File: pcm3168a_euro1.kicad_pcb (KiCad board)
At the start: 2 copper layers, 196 x 128.4 mm, 213 parts, among them J1 Conn_02x04_Odd_Even, J10 Conn_Coaxial, J11 Conn_Coaxial, J12 Conn_Coaxial, J13 Conn_Coaxial, J14 Conn_Coaxial, J15 Conn_Coaxial, J16 Conn_Coaxial, J17 ACJS-MV35-3, J18 Conn_02x08_Odd_Even, J19 Conn_Coaxial, J2 Conn_02x04_Odd_Even, J20 ACJS-MV35-3, J21 ACJS-MV35-3, J22 ACJS-MV35-3, J3 Conn_02x04_Odd_Even, J4 Conn_02x04_Odd_Even, J5 Conn_02x04_Odd_Even, J6 Conn_Coaxial, J7 Conn_Coaxial, J8 Conn_01x02_Pin, J9 Conn_Coaxial, U1 PCM3168APAPR, U10 74LVC1G17, U11 OPA1637, U12 TLV1117-33, U13 OPA1637, U14 OPA1637, U15 OPA1637, U2 74LVC1G17, U3 74LVC1G17, U4 74LVC1G17, U5 74LVC1G17, U6 74LVC1G17, U7 74LVC1G17, U8 74LVC1G17, U9 74LVC1G17, Y1 SG-210STF 24.5760ML0

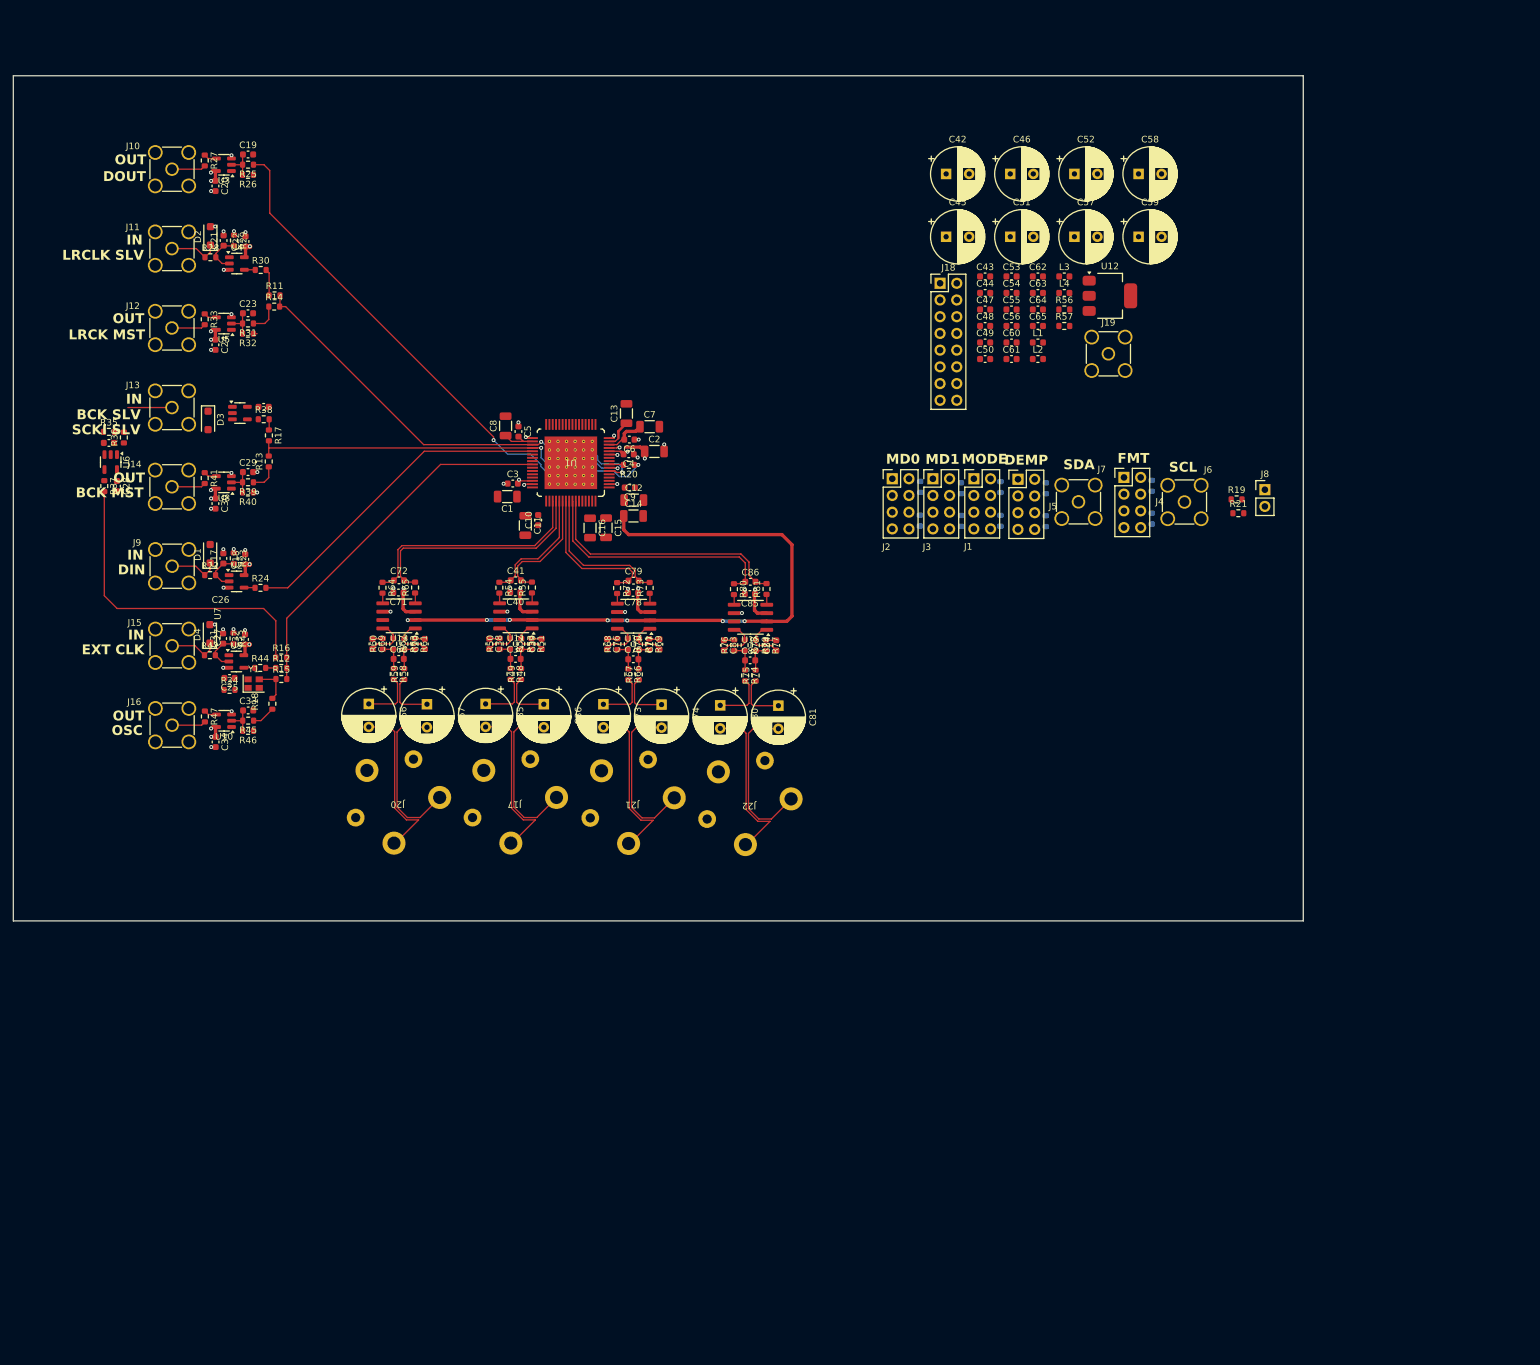
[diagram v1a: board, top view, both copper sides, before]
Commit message: WIP layout
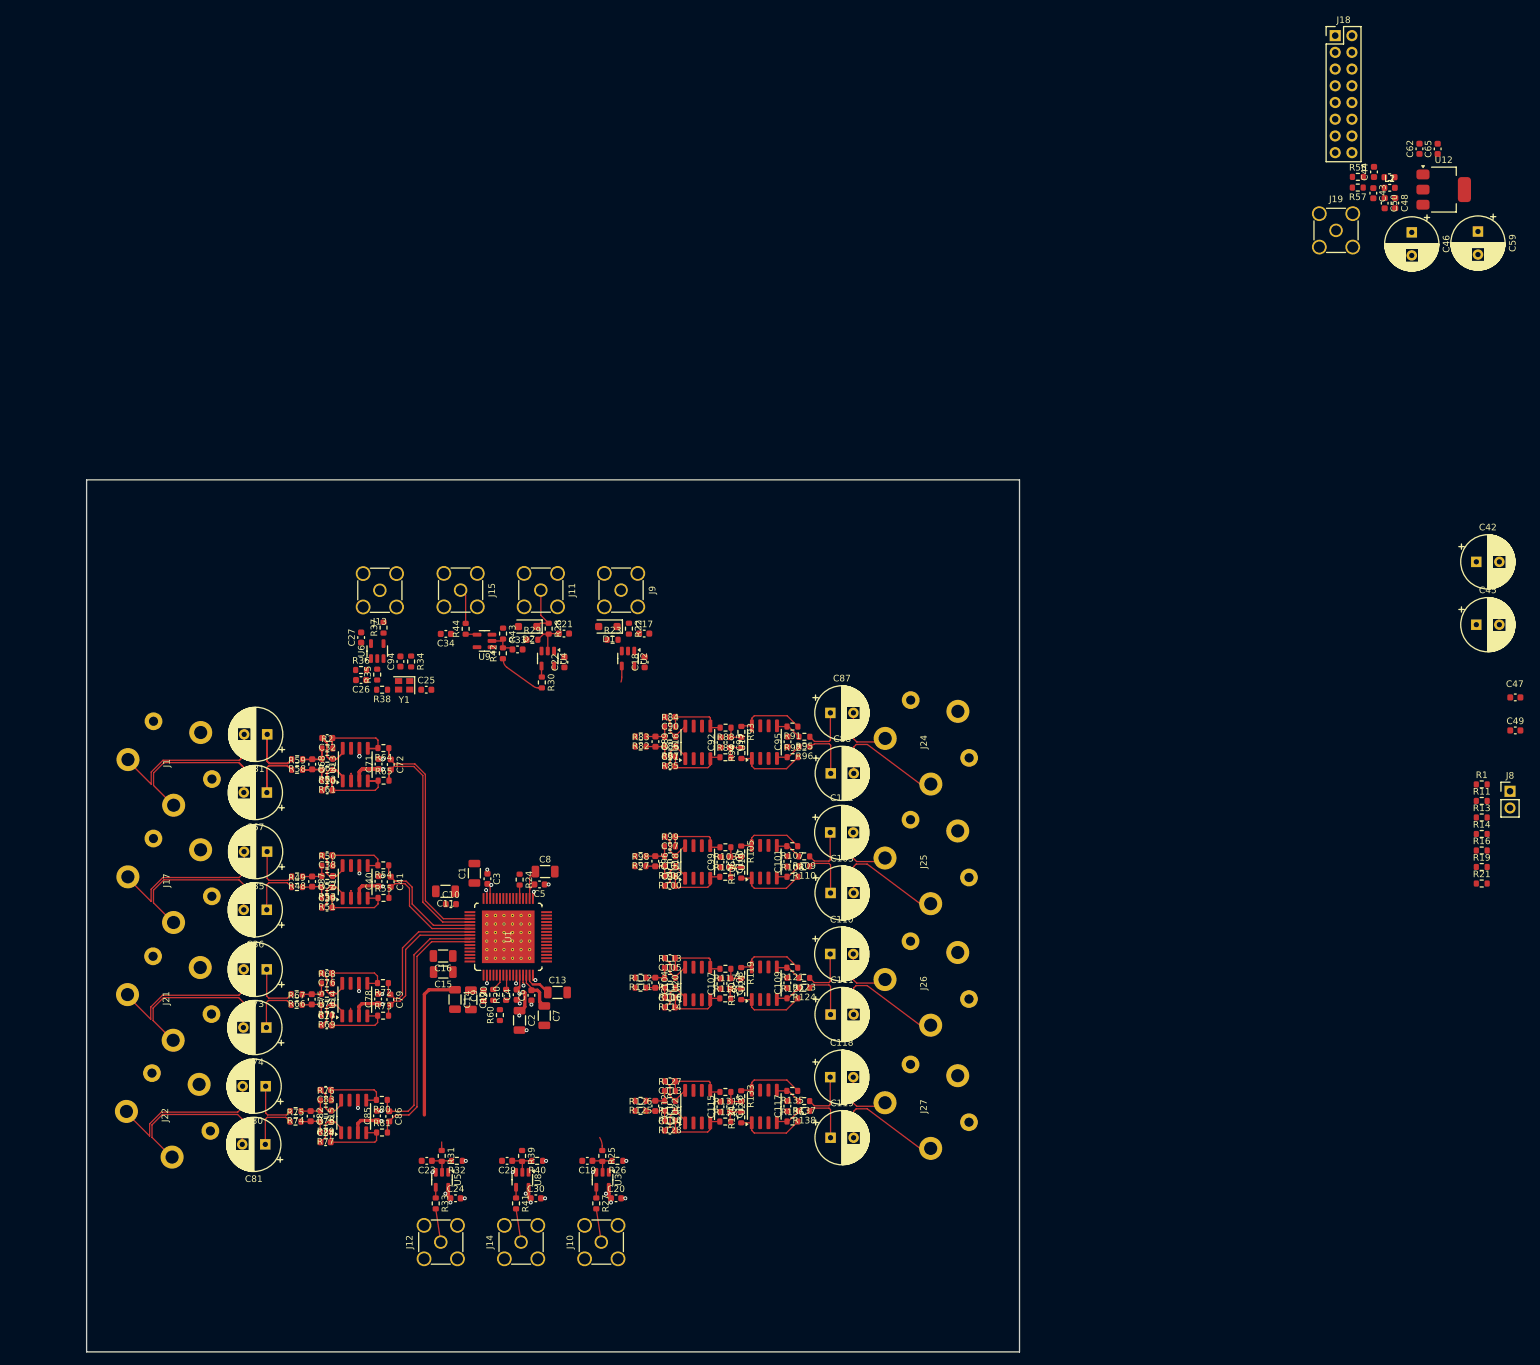
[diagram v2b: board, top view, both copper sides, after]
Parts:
- removed C28: 100nF, Capacitor_SMD:C_0603_1608Metric
- removed C51, C52, C57, C58, C66: C_Polarized_Small, Capacitor_THT:CP_Radial_D8.0mm_P3.50mm
- removed C53, C54, C55, C56, C60, C61, C63, C64: C_Small, Capacitor_SMD:C_0603_1608Metric
- removed C69: 1n, Capacitor_SMD:C_0603_1608Metric
- removed D3, D4: D_Zener_Small, Diode_SMD:D_SOD-123F
- removed J16, J6, J7: Conn_Coaxial, Connector_Coaxial:SMA_Amphenol_901-144_Vertical
- removed J2, J3, J4, J5: Conn_02x04_Odd_Even, Connector_PinHeader_2.54mm:PinHeader_2x04_P2.54mm_Vertical
- removed J20: ACJS-MV35-3, pcm3168a_euro1:Amphenol_ACJS
- removed L3, L4: L_Ferrite_Small, Inductor_SMD:L_0603_1608Metric
- removed R10, R3, R4, R5, R6, R7, R8, R9: 220k 5%, Resistor_SMD:R_0603_1608Metric
- removed R12, R15, R17, R18, R45: 0, Resistor_SMD:R_0603_1608Metric
- removed R46: R_Small, Resistor_SMD:R_0603_1608Metric
- removed R47: 22, Resistor_SMD:R_0603_1608Metric
- removed U10, U7: 74LVC1G17, Package_TO_SOT_SMD:SOT-23-5
- added C100: 39n, Capacitor_SMD:C_0603_1608Metric, F.Cu at (160.4, 142.6)
- added C101: 100nF, Capacitor_SMD:C_0603_1608Metric, F.Cu at (169.1, 142.5)
- added C102: C_Polarized_Small, Capacitor_THT:CP_Radial_D8.0mm_P3.50mm, F.Cu at (175.6, 138.1)
- added C103: C_Polarized_Small, Capacitor_THT:CP_Radial_D8.0mm_P3.50mm, F.Cu at (175.7, 147.3)
- added C104: 6.8n, Capacitor_SMD:C_0603_1608Metric, F.Cu at (149.1, 160.9)
- added C105: 1n, Capacitor_SMD:C_0603_1608Metric, F.Cu at (151.3, 157.2)
- added C106: 1n, Capacitor_SMD:C_0603_1608Metric, F.Cu at (151.3, 164.7)
- added C107: 100nF, Capacitor_SMD:C_0603_1608Metric, F.Cu at (159.0, 161.1)
- added C108: 39n, Capacitor_SMD:C_0603_1608Metric, F.Cu at (160.4, 161.0)
- added C109: 100nF, Capacitor_SMD:C_0603_1608Metric, F.Cu at (169.1, 161.0)
- added C110: C_Polarized_Small, Capacitor_THT:CP_Radial_D8.0mm_P3.50mm, F.Cu at (175.6, 156.6)
- added C111: C_Polarized_Small, Capacitor_THT:CP_Radial_D8.0mm_P3.50mm, F.Cu at (175.7, 165.8)
- added C112: 6.8n, Capacitor_SMD:C_0603_1608Metric, F.Cu at (149.1, 179.7)
- added C113: 1n, Capacitor_SMD:C_0603_1608Metric, F.Cu at (151.3, 175.9)
- added C114: 1n, Capacitor_SMD:C_0603_1608Metric, F.Cu at (151.3, 183.4)
- added C115: 100nF, Capacitor_SMD:C_0603_1608Metric, F.Cu at (159.0, 179.8)
- added C116: 39n, Capacitor_SMD:C_0603_1608Metric, F.Cu at (160.4, 179.8)
- added C117: 100nF, Capacitor_SMD:C_0603_1608Metric, F.Cu at (169.1, 179.7)
- added C118: C_Polarized_Small, Capacitor_THT:CP_Radial_D8.0mm_P3.50mm, F.Cu at (175.6, 175.3)
- added C119: C_Polarized_Small, Capacitor_THT:CP_Radial_D8.0mm_P3.50mm, F.Cu at (175.7, 184.5)
- added C87: C_Polarized_Small, Capacitor_THT:CP_Radial_D8.0mm_P3.50mm, F.Cu at (175.7, 119.9)
- added C88: C_Polarized_Small, Capacitor_THT:CP_Radial_D8.0mm_P3.50mm, F.Cu at (175.7, 129.1)
- added C89: 6.8n, Capacitor_SMD:C_0603_1608Metric, F.Cu at (149.1, 124.3)
- added C90: 1n, Capacitor_SMD:C_0603_1608Metric, F.Cu at (151.3, 120.5)
- added C91: 1n, Capacitor_SMD:C_0603_1608Metric, F.Cu at (151.3, 128.0)
- added C92: 100nF, Capacitor_SMD:C_0603_1608Metric, F.Cu at (159.0, 124.4)
- added C93: 39n, Capacitor_SMD:C_0603_1608Metric, F.Cu at (160.5, 124.4)
- added C94: 4.7uF, Capacitor_SMD:C_0603_1608Metric, F.Cu at (110.3, 112.1)
- added C95: 100nF, Capacitor_SMD:C_0603_1608Metric, F.Cu at (169.1, 124.3)
- added C96: 6.8n, Capacitor_SMD:C_0603_1608Metric, F.Cu at (149.1, 142.5)
- added C97: 1n, Capacitor_SMD:C_0603_1608Metric, F.Cu at (151.3, 138.7)
- added C98: 1n, Capacitor_SMD:C_0603_1608Metric, F.Cu at (151.3, 146.2)
- added C99: 100nF, Capacitor_SMD:C_0603_1608Metric, F.Cu at (159.0, 142.6)
- added J24: ACJS-MV35-3, pcm3168a_euro1:Amphenol_ACJS, F.Cu at (190.4, 124.4)
- added J25: ACJS-MV35-3, pcm3168a_euro1:Amphenol_ACJS, F.Cu at (190.3, 142.5)
- added J26: ACJS-MV35-3, pcm3168a_euro1:Amphenol_ACJS, F.Cu at (190.3, 161.0)
- added J27: ACJS-MV35-3, pcm3168a_euro1:Amphenol_ACJS, F.Cu at (190.3, 179.7)
- added R100: 1.1k, Resistor_SMD:R_0603_1608Metric, F.Cu at (151.3, 144.7)
- added R101: 560, Resistor_SMD:R_0603_1608Metric, F.Cu at (151.3, 141.7)
- added R102: 560, Resistor_SMD:R_0603_1608Metric, F.Cu at (151.3, 143.2)
- added R103: 47, Resistor_SMD:R_0603_1608Metric, F.Cu at (159.7, 140.3)
- added R104: 47, Resistor_SMD:R_0603_1608Metric, F.Cu at (159.7, 144.8)
- added R105: 1.1k, Resistor_SMD:R_0603_1608Metric, F.Cu at (162.1, 141.0)
- added R106: 1.1k, Resistor_SMD:R_0603_1608Metric, F.Cu at (162.1, 144.2)
- added R107: 1.1k, Resistor_SMD:R_0603_1608Metric, F.Cu at (169.9, 140.2)
- added R108: 1.1k, Resistor_SMD:R_0603_1608Metric, F.Cu at (169.9, 144.8)
- added R109: 120, Resistor_SMD:R_0603_1608Metric, F.Cu at (171.7, 141.7)
- added R110: 120, Resistor_SMD:R_0603_1608Metric, F.Cu at (171.7, 143.2)
- added R111: 1.1k, Resistor_SMD:R_0603_1608Metric, F.Cu at (146.8, 160.2)
- added R112: 1.1k, Resistor_SMD:R_0603_1608Metric, F.Cu at (146.8, 161.7)
- added R113: 1.1k, Resistor_SMD:R_0603_1608Metric, F.Cu at (151.3, 158.7)
- added R114: 1.1k, Resistor_SMD:R_0603_1608Metric, F.Cu at (151.3, 163.2)
- added R115: 560, Resistor_SMD:R_0603_1608Metric, F.Cu at (151.3, 160.2)
- added R116: 560, Resistor_SMD:R_0603_1608Metric, F.Cu at (151.3, 161.7)
- added R117: 47, Resistor_SMD:R_0603_1608Metric, F.Cu at (159.7, 158.8)
- added R118: 47, Resistor_SMD:R_0603_1608Metric, F.Cu at (159.7, 163.3)
- added R119: 1.1k, Resistor_SMD:R_0603_1608Metric, F.Cu at (162.1, 159.4)
- added R120: 1.1k, Resistor_SMD:R_0603_1608Metric, F.Cu at (162.1, 162.7)
- added R121: 1.1k, Resistor_SMD:R_0603_1608Metric, F.Cu at (169.9, 158.6)
- added R122: 1.1k, Resistor_SMD:R_0603_1608Metric, F.Cu at (169.9, 163.3)
- added R123: 120, Resistor_SMD:R_0603_1608Metric, F.Cu at (171.7, 160.2)
- added R124: 120, Resistor_SMD:R_0603_1608Metric, F.Cu at (171.7, 161.7)
- added R125: 1.1k, Resistor_SMD:R_0603_1608Metric, F.Cu at (146.8, 178.9)
- added R126: 1.1k, Resistor_SMD:R_0603_1608Metric, F.Cu at (146.8, 180.4)
- added R127: 1.1k, Resistor_SMD:R_0603_1608Metric, F.Cu at (151.3, 177.4)
- added R128: 1.1k, Resistor_SMD:R_0603_1608Metric, F.Cu at (151.3, 181.9)
- added R129: 560, Resistor_SMD:R_0603_1608Metric, F.Cu at (151.3, 178.9)
- added R130: 560, Resistor_SMD:R_0603_1608Metric, F.Cu at (151.3, 180.4)
- added R131: 47, Resistor_SMD:R_0603_1608Metric, F.Cu at (159.7, 177.5)
- added R132: 47, Resistor_SMD:R_0603_1608Metric, F.Cu at (159.7, 182.0)
- added R133: 1.1k, Resistor_SMD:R_0603_1608Metric, F.Cu at (162.1, 178.2)
- added R134: 1.1k, Resistor_SMD:R_0603_1608Metric, F.Cu at (162.1, 181.4)
- added R135: 1.1k, Resistor_SMD:R_0603_1608Metric, F.Cu at (169.9, 177.4)
- added R136: 1.1k, Resistor_SMD:R_0603_1608Metric, F.Cu at (169.9, 182.0)
- added R137: 120, Resistor_SMD:R_0603_1608Metric, F.Cu at (171.7, 178.9)
- added R138: 120, Resistor_SMD:R_0603_1608Metric, F.Cu at (171.7, 180.4)
- added R82: 1.1k, Resistor_SMD:R_0603_1608Metric, F.Cu at (146.8, 123.5)
- added R83: 1.1k, Resistor_SMD:R_0603_1608Metric, F.Cu at (146.8, 125.0)
- added R84: 1.1k, Resistor_SMD:R_0603_1608Metric, F.Cu at (151.3, 122.0)
- added R85: 1.1k, Resistor_SMD:R_0603_1608Metric, F.Cu at (151.3, 126.5)
- added R86: 560, Resistor_SMD:R_0603_1608Metric, F.Cu at (151.3, 123.5)
- added R87: 560, Resistor_SMD:R_0603_1608Metric, F.Cu at (151.3, 125.0)
- added R88: 47, Resistor_SMD:R_0603_1608Metric, F.Cu at (159.7, 122.2)
- added R89: 47, Resistor_SMD:R_0603_1608Metric, F.Cu at (159.7, 126.7)
- added R90: 22, Resistor_SMD:R_0603_1608Metric, F.Cu at (124.4, 162.8)
- added R91: 1.1k, Resistor_SMD:R_0603_1608Metric, F.Cu at (169.9, 122.0)
- added R92: 1.1k, Resistor_SMD:R_0603_1608Metric, F.Cu at (169.9, 126.7)
- added R93: 1.1k, Resistor_SMD:R_0603_1608Metric, F.Cu at (162.1, 122.8)
- added R94: 1.1k, Resistor_SMD:R_0603_1608Metric, F.Cu at (162.1, 126.0)
- added R95: 120, Resistor_SMD:R_0603_1608Metric, F.Cu at (171.7, 123.6)
- added R96: 120, Resistor_SMD:R_0603_1608Metric, F.Cu at (171.7, 125.1)
- added R97: 1.1k, Resistor_SMD:R_0603_1608Metric, F.Cu at (146.8, 141.7)
- added R98: 1.1k, Resistor_SMD:R_0603_1608Metric, F.Cu at (146.8, 143.2)
- added R99: 1.1k, Resistor_SMD:R_0603_1608Metric, F.Cu at (151.3, 140.2)
- added U16: OPA1637, Package_SO:SOIC-8_3.9x4.9mm_P1.27mm, F.Cu at (155.5, 124.4)
- added U17: OPA1637, Package_SO:SOIC-8_3.9x4.9mm_P1.27mm, F.Cu at (165.6, 124.4)
- added U18: OPA1637, Package_SO:SOIC-8_3.9x4.9mm_P1.27mm, F.Cu at (155.5, 142.6)
- added U19: OPA1637, Package_SO:SOIC-8_3.9x4.9mm_P1.27mm, F.Cu at (165.6, 142.5)
- added U20: OPA1637, Package_SO:SOIC-8_3.9x4.9mm_P1.27mm, F.Cu at (155.5, 161.0)
- added U21: OPA1637, Package_SO:SOIC-8_3.9x4.9mm_P1.27mm, F.Cu at (165.6, 161.0)
- added U22: OPA1637, Package_SO:SOIC-8_3.9x4.9mm_P1.27mm, F.Cu at (155.5, 179.8)
- added U23: OPA1637, Package_SO:SOIC-8_3.9x4.9mm_P1.27mm, F.Cu at (165.6, 179.7)
- C31: value C_Small -> C_Polarized_Small; footprint Capacitor_SMD:C_0603_1608Metric -> Capacitor_THT:CP_Radial_D8.0mm_P3.50mm
- C32: value 100nF -> 1n
- J1: value Conn_02x04_Odd_Even -> ACJS-MV35-3; footprint Connector_PinHeader_2.54mm:PinHeader_2x04_P2.54mm_Vertical -> pcm3168a_euro1:Amphenol_ACJS
- R1: moved to F.Cu
- R11, R13, R14, R16: value 0 -> 220k 5%
- R2: value 220k 5% -> 1.1k; moved to F.Cu
- R34: value 0 -> 22k
- R60: value 1.1k -> 22
- moved R14 200.2 mm to (274.6, 138.3)
- moved R11 198.9 mm to (274.6, 133.3)
- moved R13 192.1 mm to (274.6, 135.8), turned to 0 degrees
- moved R16 184.8 mm to (274.6, 140.8)
- moved J10 175.6 mm to (140.9, 200.3), turned to 90 degrees
- moved R27 169.3 mm to (140.1, 194.5)
- moved C20 165.4 mm to (143.1, 193.7), turned to 0 degrees
- moved U3 164.6 mm to (141.0, 190.9), turned to -90 degrees
- moved C19 161.4 mm to (138.7, 188.0), turned to 180 degrees
- moved R26 160.0 mm to (143.3, 188.0)
- moved R25 160.0 mm to (141.0, 187.2), turned to -90 degrees
- moved J12 144.8 mm to (116.5, 200.3), turned to 90 degrees
- moved R33 138.9 mm to (115.7, 194.5)
- moved C24 134.7 mm to (118.7, 193.7), turned to 0 degrees
- moved U5 134.3 mm to (116.6, 190.9), turned to -90 degrees
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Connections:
- C31 pad 2: GND -> Net-(J1-Pin_4)
- C32 pad 1: VDD -> Net-(C32-Pad1)
- C32 pad 2: GND -> Net-(C32-Pad2)
- C67 pad 2: Net-(J20-Pin_3) -> Net-(J1-Pin_3)
- J1 pad 1: /MODE -> GND
- J1 pad 2: GND -> unconnected-(J1-Pin_2-Pad2)
- J1 pad 3: /MODE -> Net-(J1-Pin_3)
- J1 pad 5: /MODE -> unconnected-(J1-Pin_5-Pad5)
- J13 pad 1: Net-(D3-K) -> Net-(J13-In)
- J15 pad 1: Net-(D4-K) -> Net-(J15-In)
- R1 pad 1: GND -> Net-(U1-MODE)
- R1 pad 2: Net-(J1-Pin_4) -> GND
- R11 pad 1: /lrclk_slave/OUT -> Net-(U1-MDO_ADR1_MD1)
- R11 pad 2: /LRCK -> GND
- R13 pad 1: /bck_master/IN -> VDD
- R13 pad 2: /BCK -> Net-(U1-MS_ADR0_MD0)
- R14 pad 1: /lrck_master/IN -> Net-(U1-MDI_SDA_DEMP)
- R14 pad 2: /LRCK -> GND
- R16 pad 1: /mclk/OUT1 -> VDD
- R16 pad 2: /SCKI -> Net-(U1-MC_SCL_FMT)
- R2 pad 1: GND -> Net-(C68-Pad1)
- R2 pad 2: Net-(J2-Pin_4) -> Net-(C32-Pad1)
- R30 pad 2: /lrclk_slave/OUT -> /clk_in/OUT
- R35 pad 1: Net-(D3-K) -> Net-(R35-Pad1)
- R37 pad 2: /mclk/OUT1 -> Net-(J13-In)
- R38 pad 1: Net-(R38-Pad1) -> Net-(Y1-OUT)
- R38 pad 2: /mclk/OUT2 -> Net-(R35-Pad1)
- R42 pad 1: Net-(D4-K) -> /clk_in/OUT
- R42 pad 2: Net-(C31-Pad1) -> Net-(C33-Pad1)
- R43 pad 2: Net-(C31-Pad1) -> Net-(C33-Pad1)
- R44 pad 2: /external_clock/OUT -> Net-(J15-In)
- R58 pad 2: Net-(C66-Pad1) -> Net-(C31-Pad1)
- R60 pad 1: Net-(C68-Pad1) -> /bck_master/IN
- R60 pad 2: Net-(C69-Pad1) -> Net-(U1-BCKAD)
- R62 pad 1: Net-(C69-Pad2) -> Net-(C32-Pad2)
- R64 pad 2: Net-(C69-Pad1) -> Net-(C32-Pad1)
- U1 pad 25: unconnected-(U1-VOUT4+-Pad25) -> /VOUT4+
- U1 pad 26: unconnected-(U1-VOUT4--Pad26) -> /VOUT4-
- U1 pad 27: unconnected-(U1-VOUT3+-Pad27) -> /VOUT3+
- U1 pad 28: unconnected-(U1-VOUT3--Pad28) -> /VOUT3-
- U1 pad 29: unconnected-(U1-VOUT2+-Pad29) -> /VOUT2+
- U1 pad 30: unconnected-(U1-VOUT2--Pad30) -> /VOUT2-
- U1 pad 31: unconnected-(U1-VOUT1+-Pad31) -> /VOUT1+
- U1 pad 32: unconnected-(U1-VOUT1--Pad32) -> /VOUT1-
- U1 pad 35: /LRCK -> /lrck_master/IN
- U1 pad 36: /BCK -> /bck_master/IN
- U1 pad 41: /SCKI -> /clk_in/OUT
- U1 pad 42: /FMT_SCL -> Net-(U1-MC_SCL_FMT)
- U1 pad 43: /DEMP_SDA -> Net-(U1-MDI_SDA_DEMP)
- U1 pad 44: /MD1 -> Net-(U1-MDO_ADR1_MD1)
- U1 pad 45: /MD0 -> Net-(U1-MS_ADR0_MD0)
- U1 pad 48: /MODE -> Net-(U1-MODE)
- U1 pad 6: /LRCK -> Net-(U1-LRCKAD)
- U1 pad 7: /BCK -> Net-(U1-BCKAD)
- U13 pad 5: Net-(C69-Pad1) -> Net-(C32-Pad1)
- U13 pad 8: Net-(C69-Pad2) -> Net-(C32-Pad2)
- U9 pad 2: Net-(C31-Pad1) -> Net-(C33-Pad1)
- Y1 pad 3: /oscillator/OSC_OUT -> Net-(Y1-OUT)
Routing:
- net /dout1/IN: track 83.7 -> 2.04 mm, vias 2 -> 0
- net VCOMAD: track 100.6 -> 26.8 mm, vias 7 -> 0
- net /LRCK: track 67.9 -> 0.00 mm, vias 2 -> 0
- net /BCK: track 58.8 -> 0.00 mm, vias 2 -> 0
- net /SCKI: track 56.3 -> 0.00 mm
- net /mclk/OUT1: track 49.0 -> 0.00 mm
- net /din1/OUT: track 49.1 -> 2.04 mm
- net Net-(J1-Pin_4): track 0.00 -> 29.7 mm
- net Net-(J1-Pin_3): track 0.00 -> 29.5 mm
- net Net-(J20-Pin_4): track 25.4 -> 0.00 mm
- net Net-(J20-Pin_3): track 24.7 -> 0.00 mm
- net Net-(J25-Pin_3): track 0.00 -> 16.8 mm
- net Net-(J24-Pin_3): track 0.00 -> 16.8 mm
- net Net-(J26-Pin_3): track 0.00 -> 16.8 mm
- net Net-(J27-Pin_3): track 0.00 -> 16.8 mm
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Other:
- board size 196 x 128.4 mm -> 141.8 x 132.5 mm
- board text removed: "BCK MST"
- board text removed: "BCK SLV"
- board text removed: "DEMP"
- board text removed: "DIN"
- board text removed: "DOUT"
- board text removed: "EXT CLK"
- board text removed: "FMT"
- board text removed: "IN"
- board text removed: "LRCK MST"
- board text removed: "LRCLK SLV"
- board text removed: "MD0"
- board text removed: "MD1"
- board text removed: "MODE"
- board text removed: "OSC"
- board text removed: "OUT"
- board text removed: "SCKI SLV"
- board text removed: "SCL"
- board text removed: "SDA"
